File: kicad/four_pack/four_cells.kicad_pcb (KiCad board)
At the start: 2 copper layers, 80 x 81 mm, 35 parts, among them J1 cell_+, J10 bal_even_right, J11 bal_odd_right, J12 cell_+, J13 cell_+, J14 bal_odd_right, J15 bal_even_right, J2 cell_-, J3 bal_even_left, J4 bal_even_right, J5 bal_odd_left, J6 bal_odd_right, J7 cell_+, J8 bal_odd_right, J9 bal_even_right

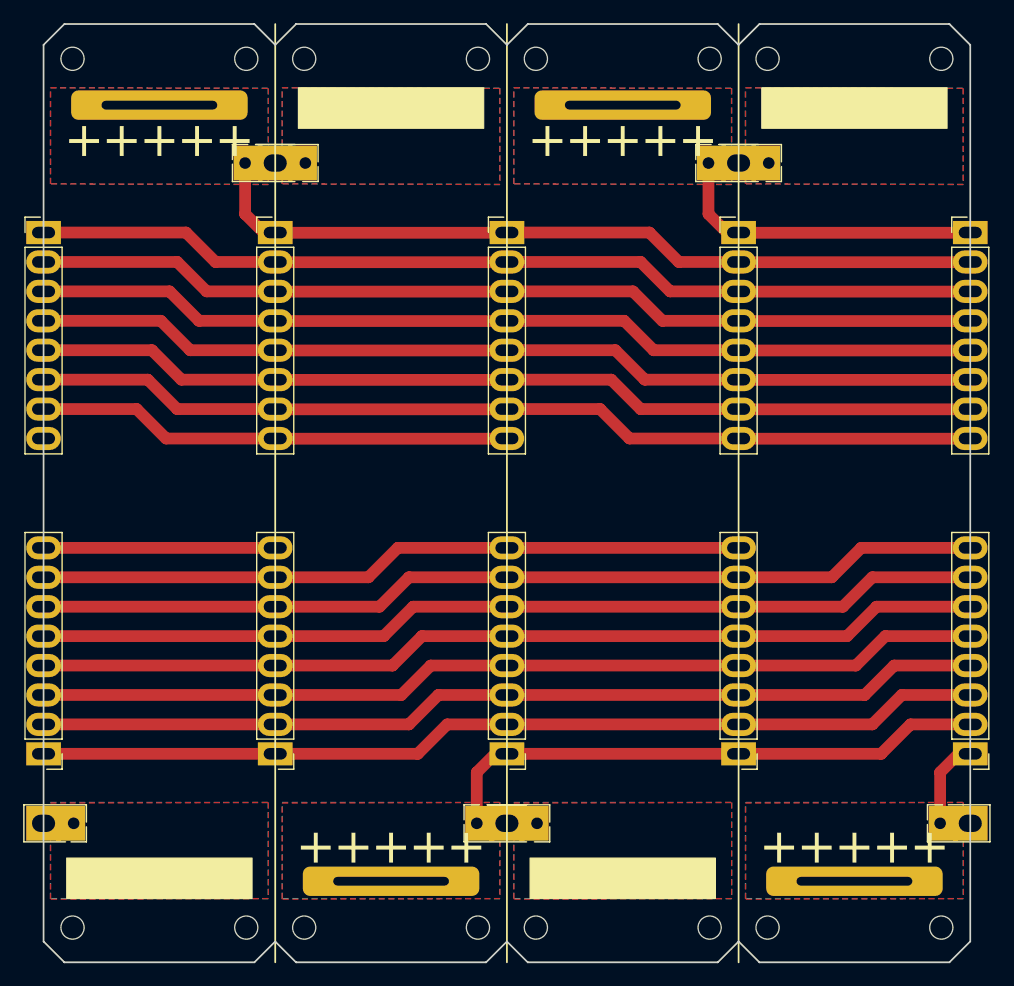
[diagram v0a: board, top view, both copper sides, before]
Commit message: Small change
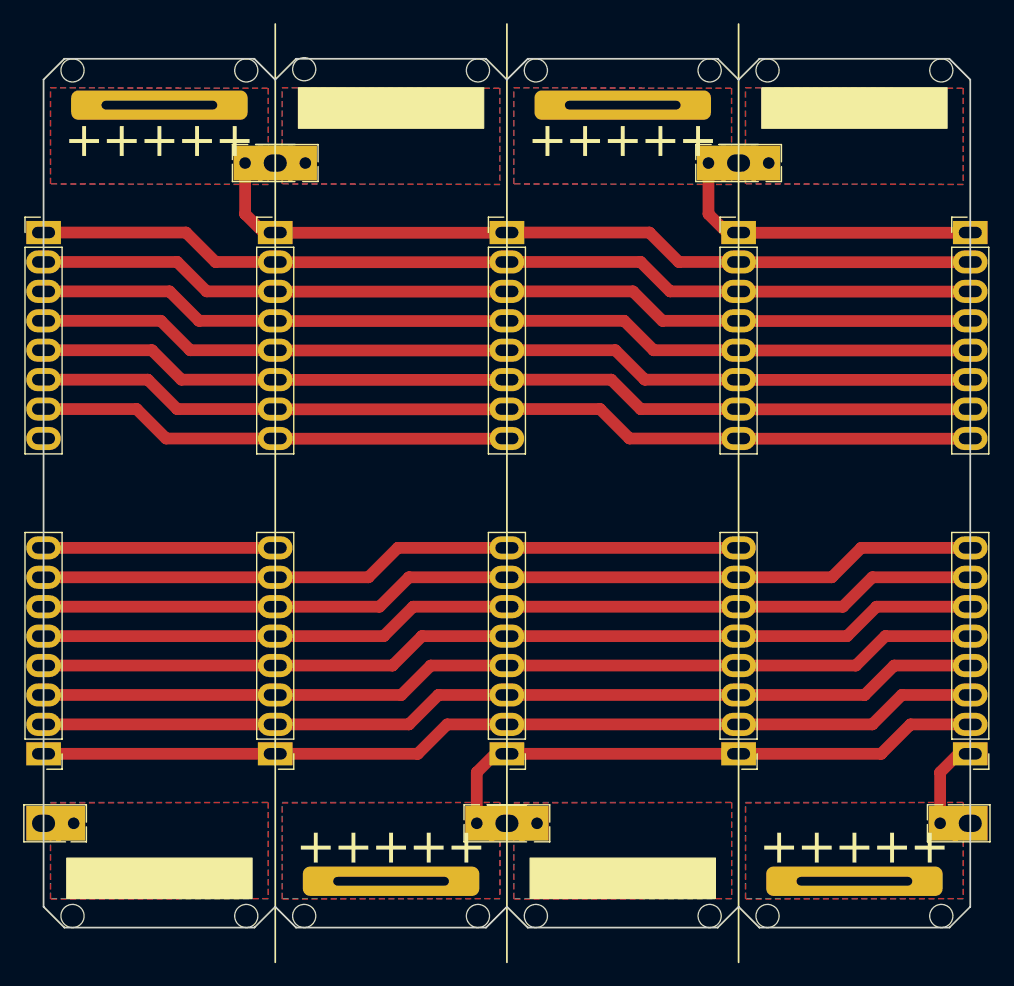
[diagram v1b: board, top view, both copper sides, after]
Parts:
- moved H1 1.00 mm to (14.5, 16.0)
- moved H10 1.00 mm to (69.5, 16.0)
- moved H11 1.00 mm to (54.5, 89.0)
- moved H12 1.00 mm to (69.5, 89.0)
- moved H13 1.00 mm to (74.5, 16.0)
- moved H14 1.00 mm to (89.5, 16.0)
- moved H15 1.00 mm to (74.5, 89.0)
- moved H16 1.00 mm to (89.5, 89.0)
- moved H2 1.00 mm to (29.5, 16.0)
- moved H3 1.00 mm to (29.5, 89.0)
- moved H4 1.00 mm to (14.5, 89.0)
- moved H6 1.00 mm to (49.5, 16.0)
- moved H7 1.00 mm to (34.5, 89.0)
- moved H8 1.00 mm to (49.5, 89.0)
- moved H9 1.00 mm to (54.5, 16.0)
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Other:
- board size 80 x 81 mm -> 80 x 75 mm
